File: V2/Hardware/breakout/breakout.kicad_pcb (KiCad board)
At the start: 2 copper layers, 8 parts, among them J0 Flat_7seg_F, J1 Conn_D, J2 Conn_C, J3 Conn_E, J4 Conn_B, J5 Conn_F, J6 Conn_A, J7 Conn_G

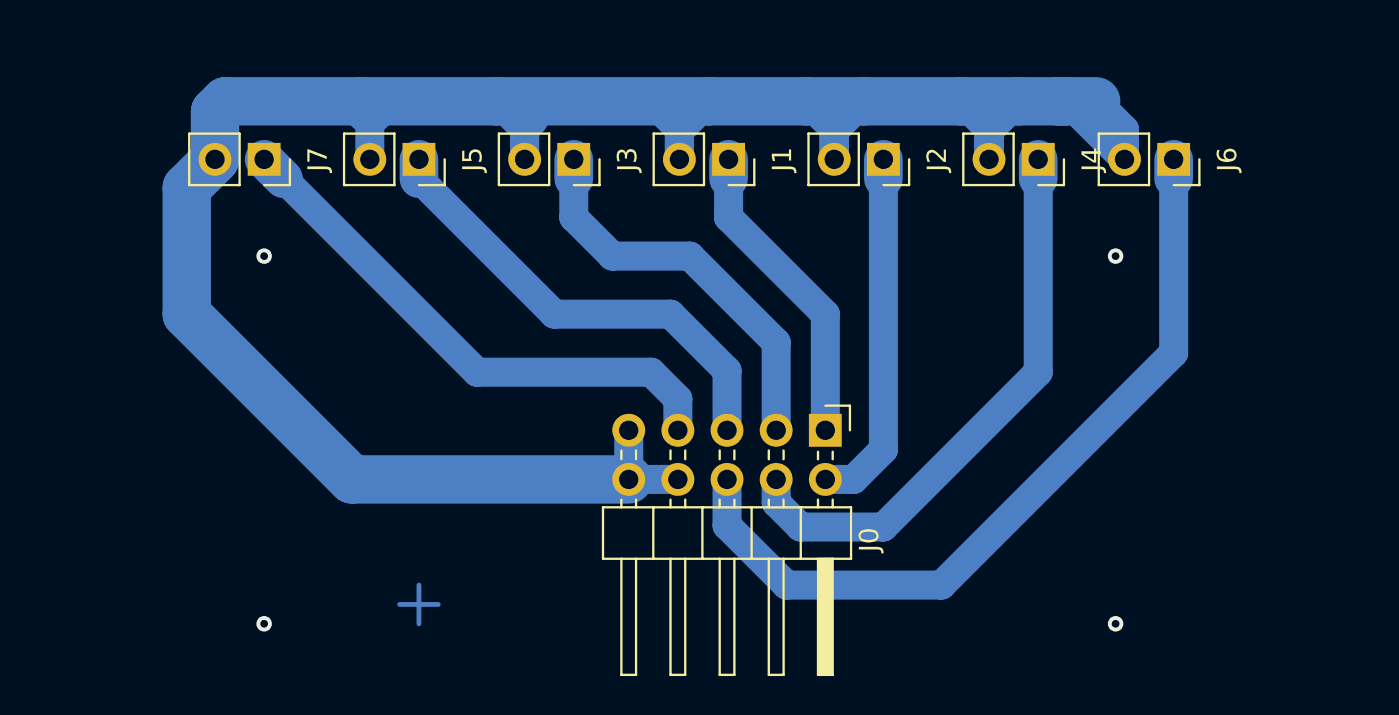
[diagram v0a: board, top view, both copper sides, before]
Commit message: revision 2 boards
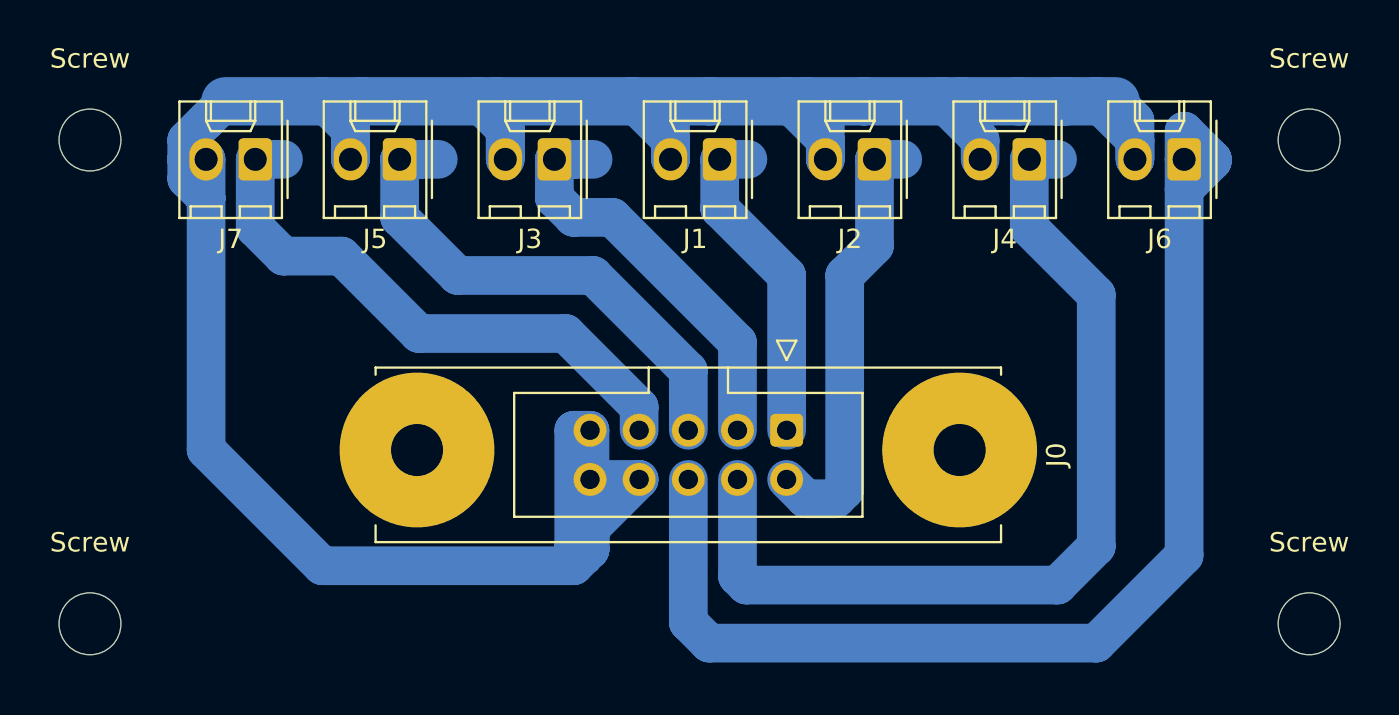
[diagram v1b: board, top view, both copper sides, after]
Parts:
- added Screw: MountingHole_3.2mm_M3, MountingHole:MountingHole_3.2mm_M3, F.Cu at (190.0, 86.0)
- added Screw: MountingHole_3.2mm_M3, MountingHole:MountingHole_3.2mm_M3, F.Cu at (190.0, 61.0)
- added Screw: MountingHole_3.2mm_M3, MountingHole:MountingHole_3.2mm_M3, F.Cu at (127.0, 86.0)
- added Screw: MountingHole_3.2mm_M3, MountingHole:MountingHole_3.2mm_M3, F.Cu at (127.0, 61.0)
- J0: value Flat_7seg_F -> 7SEG_12V; footprint Connector_PinHeader_2.54mm:PinHeader_2x05_P2.54mm_Horizontal -> Connector_IDC:IDC-Header_2x05-1MP_P2.54mm_Latch_Vertical
- J1, J2, J3, J4, J5, J6, J7: footprint Connector_PinSocket_2.54mm:PinSocket_1x02_P2.54mm_Vertical -> Connector_Molex:Molex_KK-254_AE-6410-02A_1x02_P2.54mm_Vertical
- moved J0 2.00 mm to (163.0, 76.0)
- moved J3 1.00 mm to (151.0, 62.0), turned to 180 degrees
- moved J5 1.00 mm to (143.0, 62.0), turned to 180 degrees
- moved J6 0.54 mm to (183.5, 62.0), turned to 180 degrees
- moved J1 0.46 mm to (159.5, 62.0), turned to 180 degrees
- moved J2 0.46 mm to (167.5, 62.0), turned to 180 degrees
- moved J4 0.46 mm to (175.5, 62.0), turned to 180 degrees
- moved J7 0.46 mm to (135.5, 62.0), turned to 180 degrees
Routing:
- net /SEG_A: track 41.7 -> 62.9 mm
- net /SEG_B: track 29.6 -> 47.5 mm
- net /+12V: track 180.8 -> 194.5 mm
- net /SEG_C: track 18.6 -> 22.8 mm
- net (no net): track 4.00 -> 0.00 mm, vias 4 -> 0
- net /SEG_F: track 24.1 -> 27.3 mm
- net /SEG_G: track 28.1 -> 29.9 mm
- net /SEG_E: track 20.7 -> 22.1 mm
- net /SEG_D: track 16.1 -> 16.9 mm
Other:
- board text added: "33 mm"
- board text added: "71 mm"
- board text removed: "33mm"
- board text removed: "56mm"
